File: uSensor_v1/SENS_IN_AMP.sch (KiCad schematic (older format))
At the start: 8 parts

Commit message: Schematic in progress.
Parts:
- U?: footprint Package_TO_SOT_SMD:TSOT-23-5 -> (none)
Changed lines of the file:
@@
 F 0 "U?" H 5500 3650 50  0000 L CNN
 F 1 "LM6132A/NS" H 5650 3650 50  0000 L CNN
-F 2 "Package_TO_SOT_SMD:TSOT-23-5" H 5400 3550 50  0001 C CNN
+F 2 "" H 5400 3550 50  0001 C CNN
 F 3 "http://www.analog.com/media/en/technical-documentation/data-sheets/AD8603_8607_8609.pdf" H 5400 3750 50  0001 C CNN
 	1    5400 3550
@@
 AR Path="/5C86721C/5C6F0253" Ref="C?"  Part="1"
 AR Path="/5C829D40/5C6F0253" Ref="C?"  Part="1"
+AR Path="/5C7ECB16/5C6F0253" Ref="C?"  Part="1"
 F 0 "C?" H 6115 2946 50  0000 L CNN
 F 1 "100n 6V3 X5R" H 6115 2855 50  0000 L CNN

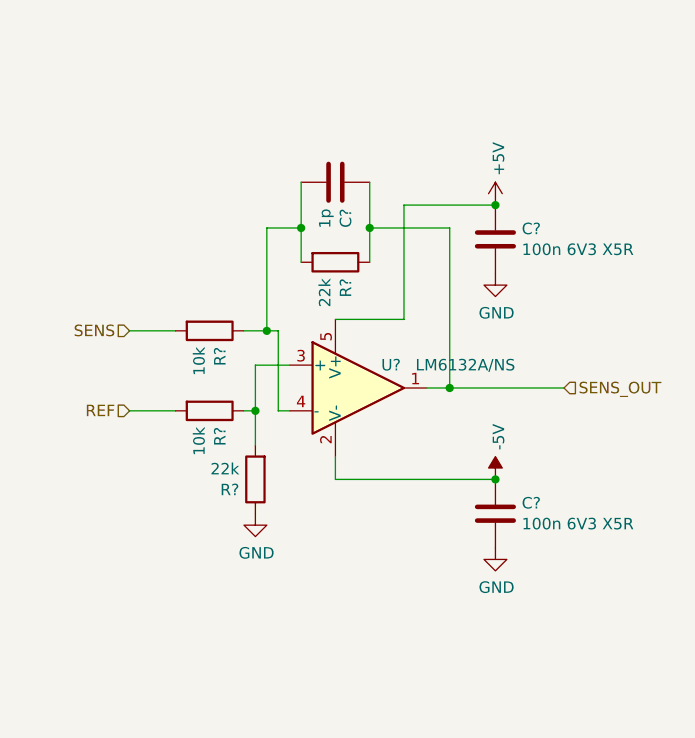
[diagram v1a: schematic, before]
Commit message: Schematic in progress.
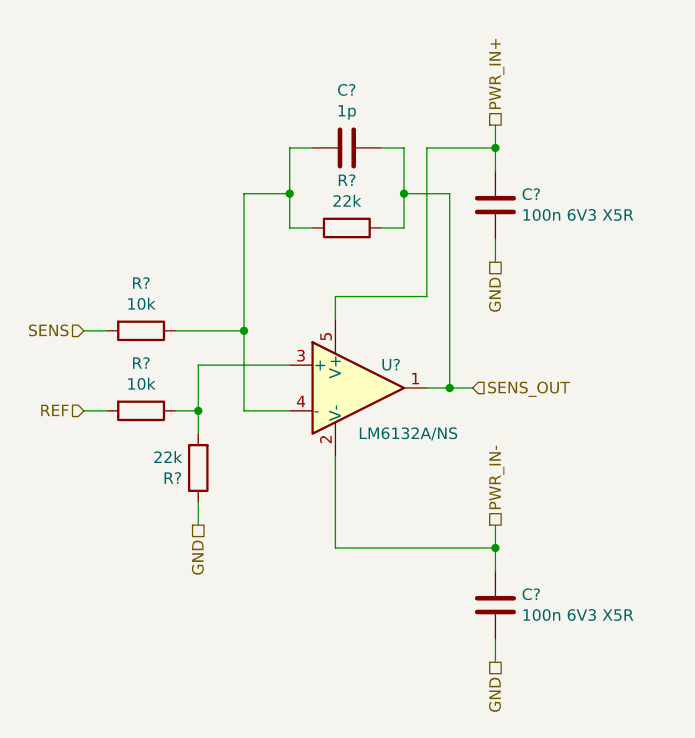
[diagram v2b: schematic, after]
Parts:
- C? (x3): footprint (none) -> Capacitor_SMD:C_0603_1608Metric_Pad1.05x0.95mm_HandSolder
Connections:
- net +5V renamed PWR_IN+
- net -5V renamed PWR_IN-
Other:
- moved on the sheet: C?, R?
